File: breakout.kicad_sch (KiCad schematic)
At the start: 1 part, among them J34 Conn_02x08_Odd_Even

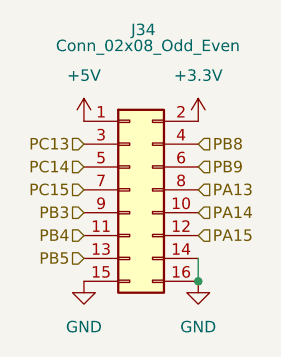
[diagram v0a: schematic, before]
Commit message: lots🅿️
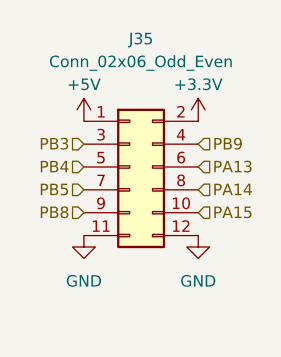
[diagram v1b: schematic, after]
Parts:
- removed J34: Conn_02x08_Odd_Even, symbol Connector_Generic:Conn_02x08_Odd_Even
- added J35: Conn_02x06_Odd_Even, Connector_PinHeader_2.54mm:PinHeader_2x06_P2.54mm_Vertical, symbol Connector_Generic:Conn_02x06_Odd_Even
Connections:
- net +3.3V: now also J35.2 (Pin_2)
- net +5V: now also J35.1 (Pin_1)
- net GND: now also J35.11 (Pin_11), J35.12 (Pin_12)
- net PA13: now also J35.6 (Pin_6)
- net PA14: now also J35.8 (Pin_8)
- net PA15: now also J35.10 (Pin_10)
- net PB3: now also J35.3 (Pin_3)
- net PB4: now also J35.5 (Pin_5)
- net PB5: now also J35.7 (Pin_7)
- net PB8: now also J35.9 (Pin_9)
- net PB9: now also J35.4 (Pin_4)

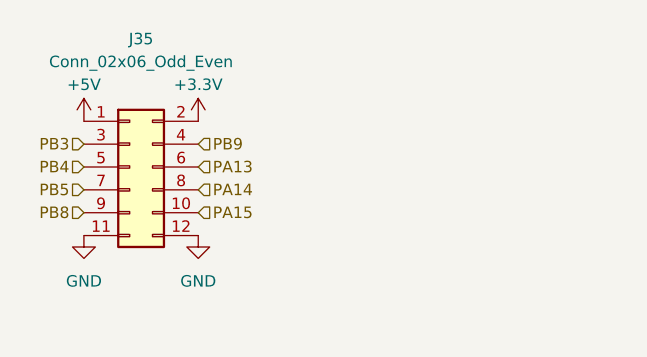
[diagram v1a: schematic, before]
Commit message: done ✅
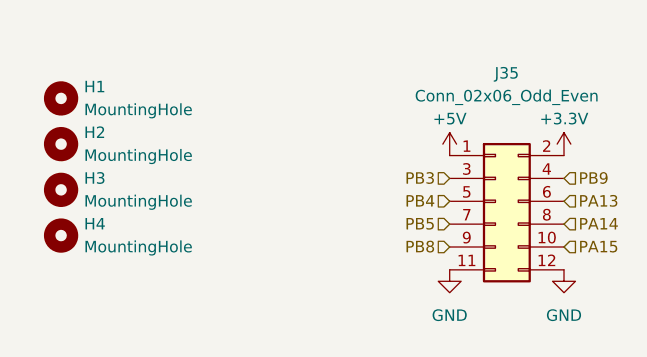
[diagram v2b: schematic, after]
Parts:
- added H1, H2, H3, H4: MountingHole, MountingHole:MountingHole_2.2mm_M2_DIN965_Pad, symbol Mechanical:MountingHole
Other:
- moved on the sheet: J35

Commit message: First Draft of BOM
Didn't select some compoentns like diodes that I don't fully understand. Also, some components have multiple variants so we must be careful.
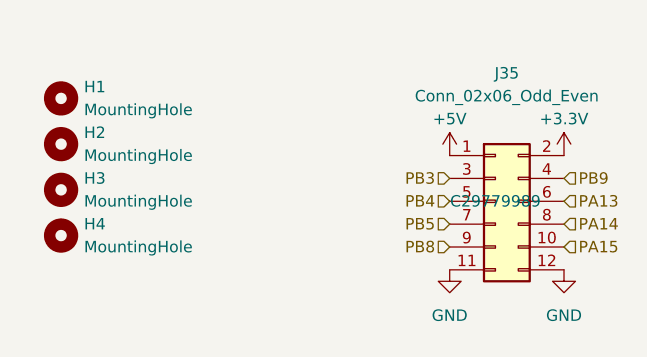
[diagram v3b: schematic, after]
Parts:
- J35: JLC# (none) -> C29779989
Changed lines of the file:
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@@
+			)
+		)
+		(property "JLC#" ""
+			(at 100.33 87.63 0)
+			(effects
+				(font
+					(size 1.27 1.27)
+				)
 			)
 		)
@@
 			)
 		)
+		(property "JLC#" ""
+			(at 100.33 92.71 0)
+			(effects
+				(font
+					(size 1.27 1.27)
+				)
+			)
+		)
 		(instances
 			(project "Alpha_Breakout"
@@
 			)
 		)
+		(property "JLC#" ""
+			(at 100.33 82.55 0)
+			(effects
+				(font
+					(size 1.27 1.27)
+				)
+			)
+		)
 		(instances
 			(project ""
@@
 				)
 				(hide yes)
+			)
+		)
+		(property "JLC#" "C29779989"
+			(at 148.59 93.98 0)
+			(effects
+				(font
+					(size 1.27 1.27)
+				)
 			)
 		)
@@
 			)
 		)
+		(property "JLC#" ""
+			(at 100.33 97.79 0)
+			(effects
+				(font
+					(size 1.27 1.27)
+				)
+			)
+		)

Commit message: parts⚙️
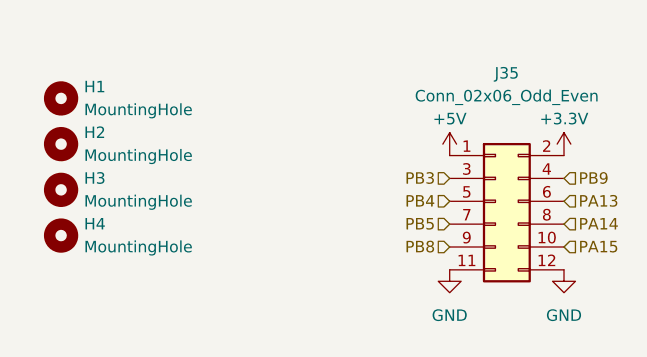
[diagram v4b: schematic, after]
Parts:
- J35: JLC# C29779989 -> (none)
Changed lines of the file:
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@@
-			)
-		)
-		(property "JLC#" "C29779989"
-			(at 148.59 93.98 0)
-			(effects
-				(font
-					(size 1.27 1.27)
-				)
 			)
 		)
